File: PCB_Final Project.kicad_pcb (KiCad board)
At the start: 2 copper layers, 29 parts, among them J1 Conn_01x02_Socket, J2 Conn_01x02_Pin, J3 Conn_01x02_Socket, K1 Relay_SPDT, K2 Relay_SPDT, Q1 NPN, Q2 NPN, U1 WeMos_D1_mini, U2 PC817, U3 PC817

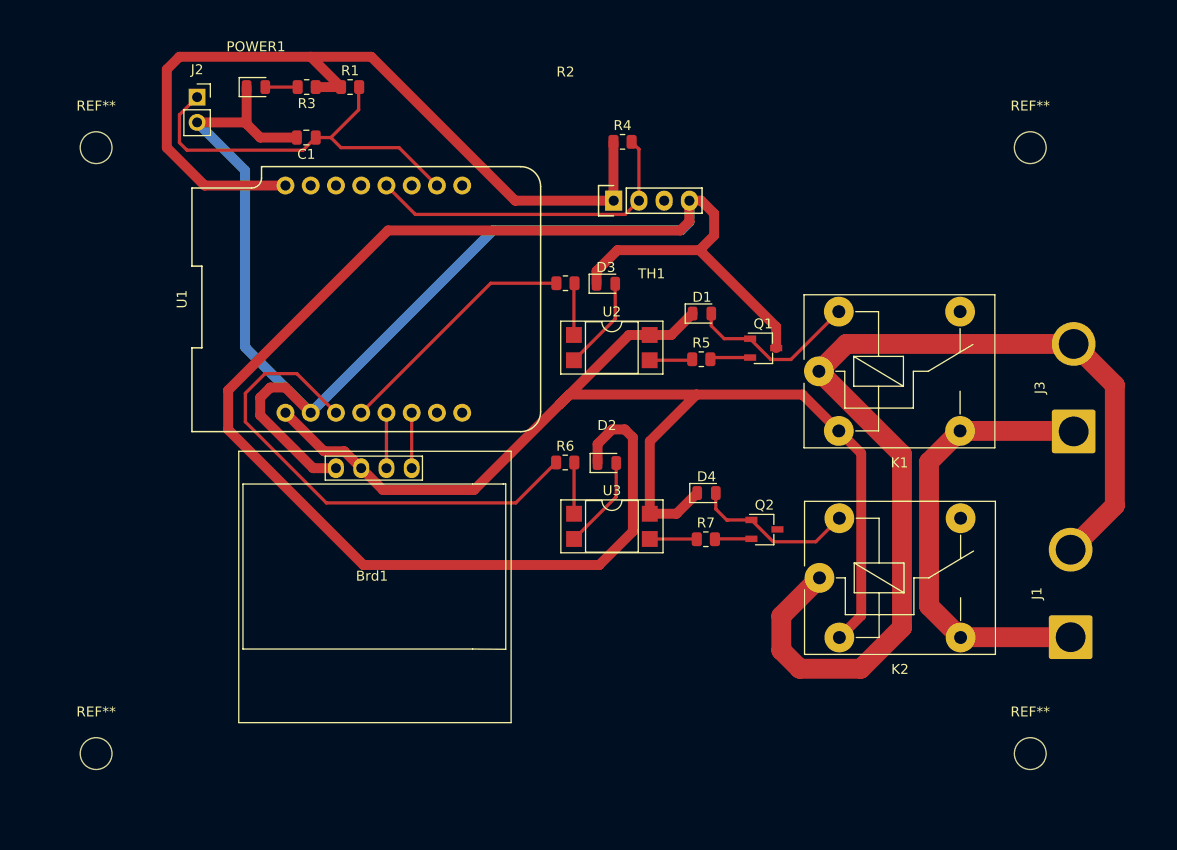
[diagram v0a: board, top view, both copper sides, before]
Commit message: small correction on pcb
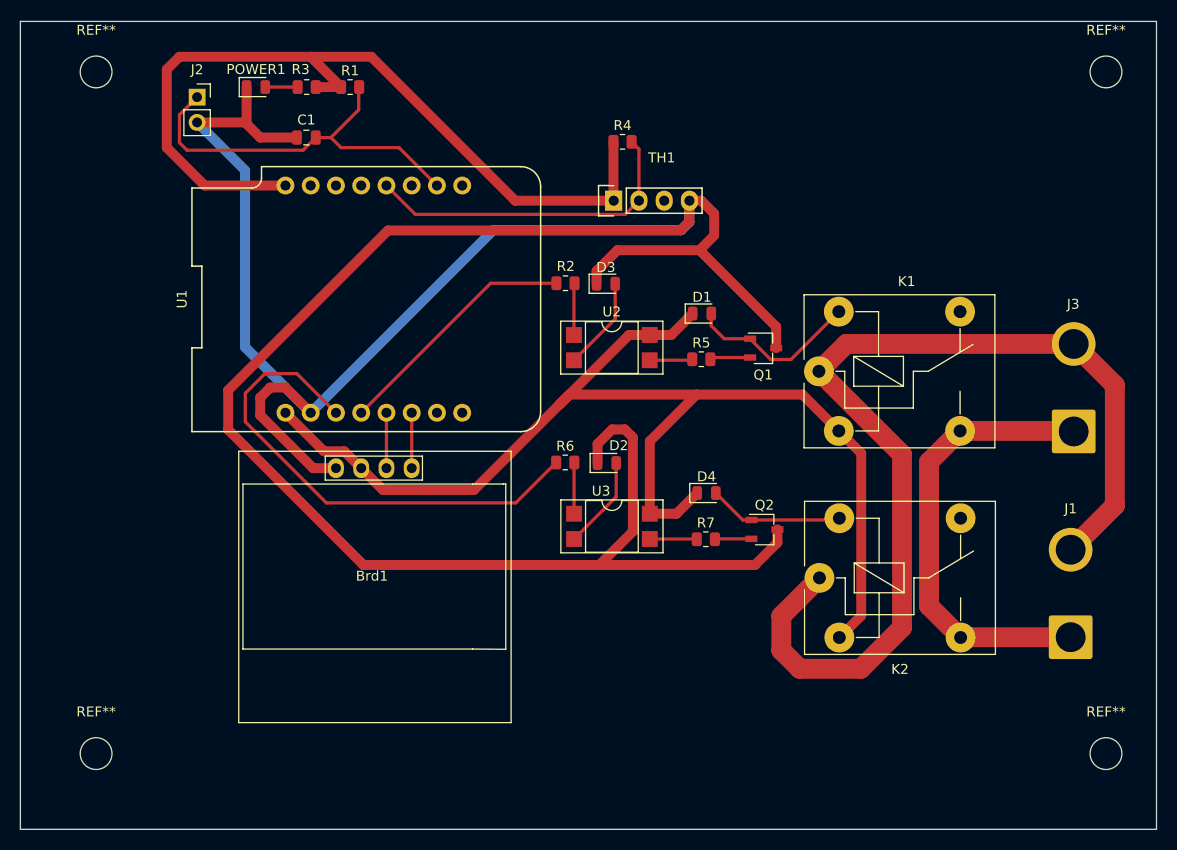
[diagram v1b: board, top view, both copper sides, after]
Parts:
- moved REF** 10.8 mm to (134.6, 53.3)
- moved REF** 7.62 mm to (134.6, 121.9)
- moved REF** 7.62 mm to (33.0, 53.3)
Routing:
- net GND: track 270.7 -> 290.9 mm
- net Net-(D4-A): track 16.4 -> 13.6 mm
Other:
- board outline added: 114.3 x 81.3 mm
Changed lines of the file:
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@@
     (property "ki_keywords" "Single Pole Relay SPDT")
     (attr through_hole)
-    (fp_text reference "K1" (at 8.1 9.2) (layer "F.SilkS")
-        (effects (font (size 1 1) (thickness 0.15)))
-    )
-    (fp_text value "Relay_SPDT" (at 8 -9.6) (layer "F.Fab")
+    (fp_text reference "K1" (at 8.8152 -9.0368) (layer "F.SilkS")
+        (effects (font (size 1 1) (thickness 0.15)))
+    )
+    (fp_text value "Relay_SPDT" (at 8.3072 0.1072) (layer "F.Fab")
         (effects (font (size 1 1) (thickness 0.15)))
     )
@@
     (property "ki_keywords" "cap capacitor")
     (attr smd)
-    (fp_text reference "C1" (at 0 -1.68) (layer "F.SilkS")
+    (fp_text reference "C1" (at 0 1.778) (layer "F.SilkS")
         (effects (font (size 1 1) (thickness 0.15)))
     )
@@
     (property "ki_keywords" "R res resistor")
     (attr smd)
-    (fp_text reference "R3" (at 0 -1.65) (layer "F.SilkS")
+    (fp_text reference "R3" (at 0.6115 1.778) (layer "F.SilkS")
         (effects (font (size 1 1) (thickness 0.15)))
     )
@@
   )
   (footprint "MountingHole:MountingHole_3.2mm_M3" (layer "F.Cu")
-    (at 127 60.96)
+    (at 134.62 53.34)
     (descr "Mounting Hole 3.2mm, no annular, M3")
     (tags "mounting hole 3.2mm no annular m3")
@@
     (property "ki_keywords" "R res resistor")
     (attr smd)
-    (fp_text reference "R2" (at 0 -21.2598) (layer "F.SilkS")
+    (fp_text reference "R2" (at 0.0235 -1.7018) (layer "F.SilkS")
         (effects (font (size 1 1) (thickness 0.15)))
     )
@@
     (property "ki_keywords" "DHT22, temperature, humidity")
     (attr through_hole)
-    (fp_text reference "TH1" (at 0 7.35) (layer "F.SilkS")
+    (fp_text reference "TH1" (at 1.016 -4.318) (layer "F.SilkS")
         (effects (font (size 1 1) (thickness 0.15)))
     )
@@
     (property "ki_keywords" "connector")
     (attr exclude_from_pos_files)
-    (fp_text reference "J1" (at 4.4 -3.4 90) (layer "F.SilkS")
+    (fp_text reference "J1" (at 12.9286 0) (layer "F.SilkS")
         (effects (font (size 1 1) (thickness 0.15)))
     )
@@
     (property "ki_keywords" "LED diode")
     (attr smd)
-    (fp_text reference "POWER1" (at 0 -4.064) (layer "F.SilkS")
+    (fp_text reference "POWER1" (at 0 -1.778) (layer "F.SilkS")
         (effects (font (size 1 1) (thickness 0.15)))
     )
@@
   )
   (footprint "MountingHole:MountingHole_3.2mm_M3" (layer "F.Cu")
-    (at 33.02 60.96)
+    (at 33.02 53.34)
     (descr "Mounting Hole 3.2mm, no annular, M3")
     (tags "mounting hole 3.2mm no annular m3")
@@
   )
   (footprint "MountingHole:MountingHole_3.2mm_M3" (layer "F.Cu")
-    (at 127 121.92)
+    (at 134.62 121.92)
     (descr "Mounting Hole 3.2mm, no annular, M3")
     (tags "mounting hole 3.2mm no annular m3")
@@
     (property "ki_keywords" "connector")
     (attr exclude_from_pos_files)
-    (fp_text reference "J3" (at 4.4 -3.4 90) (layer "F.SilkS")
+    (fp_text reference "J3" (at 12.8016 -0.0508) (layer "F.SilkS")
         (effects (font (size 1 1) (thickness 0.15)))
     )
@@
     (property "ki_keywords" "LED diode")
     (attr smd)
-    (fp_text reference "D2" (at 0 -3.7846) (layer "F.SilkS")
+    (fp_text reference "D2" (at 1.1915 -1.7526) (layer "F.SilkS")
         (effects (font (size 1 1) (thickness 0.15)))
     )
@@
     (property "ki_keywords" "simulation")
     (attr smd)
-    (fp_text reference "Q1" (at 0 -2.45) (layer "F.SilkS")
+    (fp_text reference "Q1" (at 0 2.6924) (layer "F.SilkS")
         (effects (font (size 1 1) (thickness 0.15)))
     )
@@
     (property "ki_keywords" "NPN DC Optocoupler")
     (attr smd)
-    (fp_text reference "U3" (at 0 -3.6) (layer "F.SilkS")
+    (fp_text reference "U3" (at -1.0922 -3.556) (layer "F.SilkS")
         (effects (font (size 1 1) (thickness 0.15)))
     )
@@
     )
   )
+  (gr_rect (start 25.4 48.26) (end 139.7 129.54)
+    (stroke (width 0.1) (type default)) (fill none) (layer "Edge.Cuts"))
   (segment (start 64.77 87.63) (end 64.77 93.206) (width 0.33) (layer "F.Cu") (net 1))
   (segment (start 62.23 87.63) (end 62.23 93.206) (width 0.33) (layer "F.Cu") (net 2))
   (segment (start 48.163 54.864) (end 48.163 58.577) (width 1) (layer "F.Cu") (net 3))
+  (segment (start 101.5638 100.6898) (end 99.3074 102.9462) (width 1) (layer "F.Cu") (net 3))
+  (segment (start 101.5638 99.3648) (end 101.5638 100.6898) (width 1) (layer "F.Cu") (net 3))
   (segment (start 57.15 93.206) (end 54.852 93.206) (width 1) (layer "F.Cu") (net 3))
   (segment (start 54.852 93.206) (end 49.53 87.884) (width 1) (layer "F.Cu") (net 3))
@@
   (segment (start 84.9376 89.3064) (end 86.2076 89.3064) (width 1) (layer "F.Cu") (net 3))
   (segment (start 87.0204 90.1192) (end 87.0204 99.568) (width 1) (layer "F.Cu") (net 3))
+  (segment (start 99.3074 102.9462) (end 83.6422 102.9462) (width 1) (layer "F.Cu") (net 3))
   (segment (start 93.9038 66.294) (end 95.1992 67.5894) (width 1) (layer "F.Cu") (net 3))
   (segment (start 95.1992 67.5894) (end 95.1992 69.7992) (width 1) (layer "F.Cu") (net 3))
@@
   (segment (start 81.0906 82.3468) (end 85.2424 78.195) (width 0.33) (layer "F.Cu") (net 16))
   (segment (start 85.2424 78.195) (end 85.2424 74.6506) (width 0.33) (layer "F.Cu") (net 16))
-  (segment (start 98.9438 98.4148) (end 101.1384 100.6094) (width 0.33) (layer "F.Cu") (net 22))
-  (segment (start 95.3662 97.322) (end 96.4946 98.4504) (width 0.33) (layer "F.Cu") (net 22))
-  (segment (start 95.3662 95.7072) (end 95.3662 97.322) (width 0.33) (layer "F.Cu") (net 22))
-  (segment (start 101.1384 100.6094) (end 105.425 100.6094) (width 0.33) (layer "F.Cu") (net 22))
-  (segment (start 96.5302 98.4148) (end 98.9438 98.4148) (width 0.33) (layer "F.Cu") (net 22))
-  (segment (start 96.4946 98.4504) (end 96.5302 98.4148) (width 0.33) (layer "F.Cu") (net 22))
-  (segment (start 105.425 100.6094) (end 107.7928 98.2416) (width 0.33) (layer "F.Cu") (net 22))
+  (segment (start 107.6196 98.4148) (end 107.7928 98.2416) (width 0.33) (layer "F.Cu") (net 22))
+  (segment (start 98.0738 98.4148) (end 98.9438 98.4148) (width 0.33) (layer "F.Cu") (net 22))
+  (segment (start 95.3662 95.7072) (end 98.0738 98.4148) (width 0.33) (layer "F.Cu") (net 22))
+  (segment (start 98.9438 98.4148) (end 107.6196 98.4148) (width 0.33) (layer "F.Cu") (net 22))
   (segment (start 131.064 110.2106) (end 120.0238 110.2106) (width 2) (layer "F.Cu") (net 23))
   (segment (start 116.8146 107.0634) (end 116.8146 92.583) (width 2) (layer "F.Cu") (net 23))
